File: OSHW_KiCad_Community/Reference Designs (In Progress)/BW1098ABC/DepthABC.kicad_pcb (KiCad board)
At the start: 4 copper layers, 150 x 65.2 mm, 118 parts, among them J1 Conn_02x05_Odd_Even, J13 DF23C-50DP-0.5V_92_, J2 FAN, J3 BW1099EMB_SoM, J4 Conn_02x05_Odd_Even, J5 USBC 3.1 Vertical, J6 26_pin_FFC, J7 26_pin_FFC, J9 26_pin_FFC, Q1 RK7002B, Q2 RK7002B, Q3 RK7002B, Q4 RK7002B, Q5 RK7002B, U1 2-bit bidirectional level shi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, U6 USB Type-C Switch, U7 USB Type-C Port Control

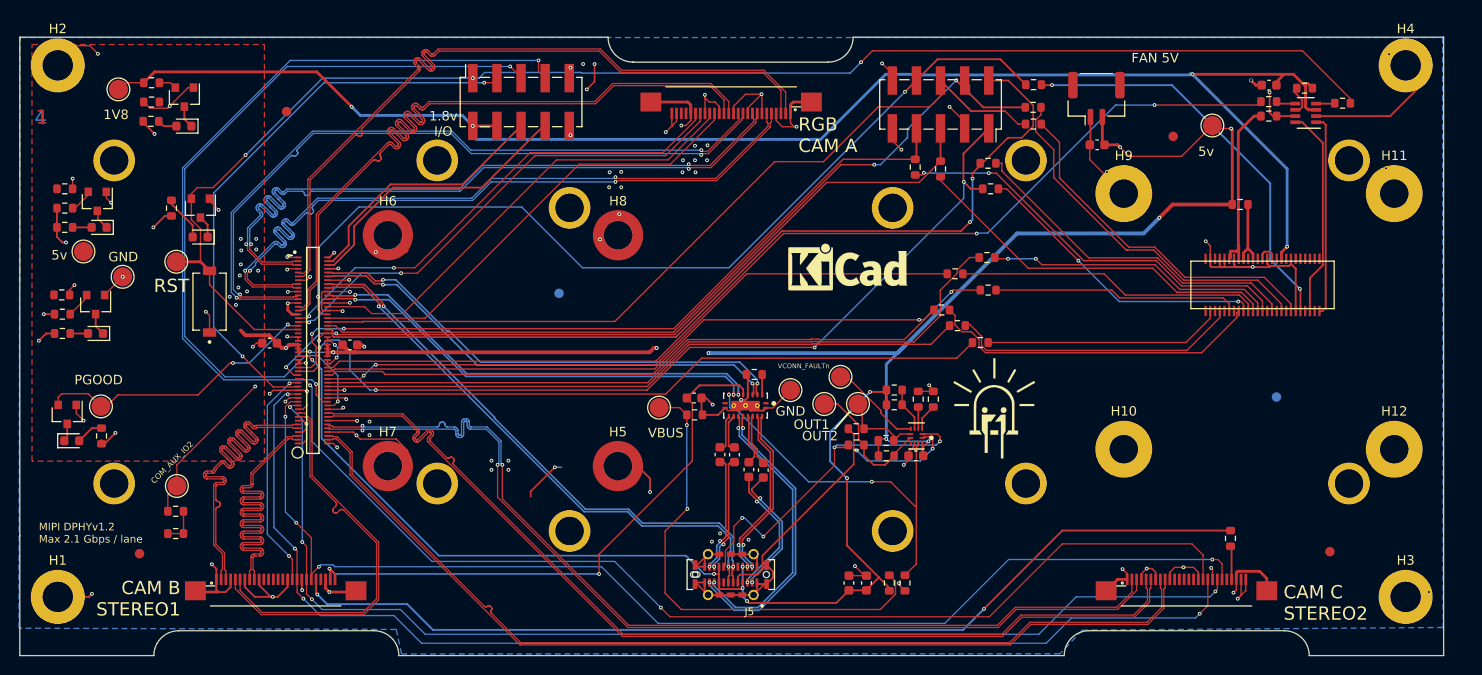
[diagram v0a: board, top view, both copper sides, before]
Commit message: skew
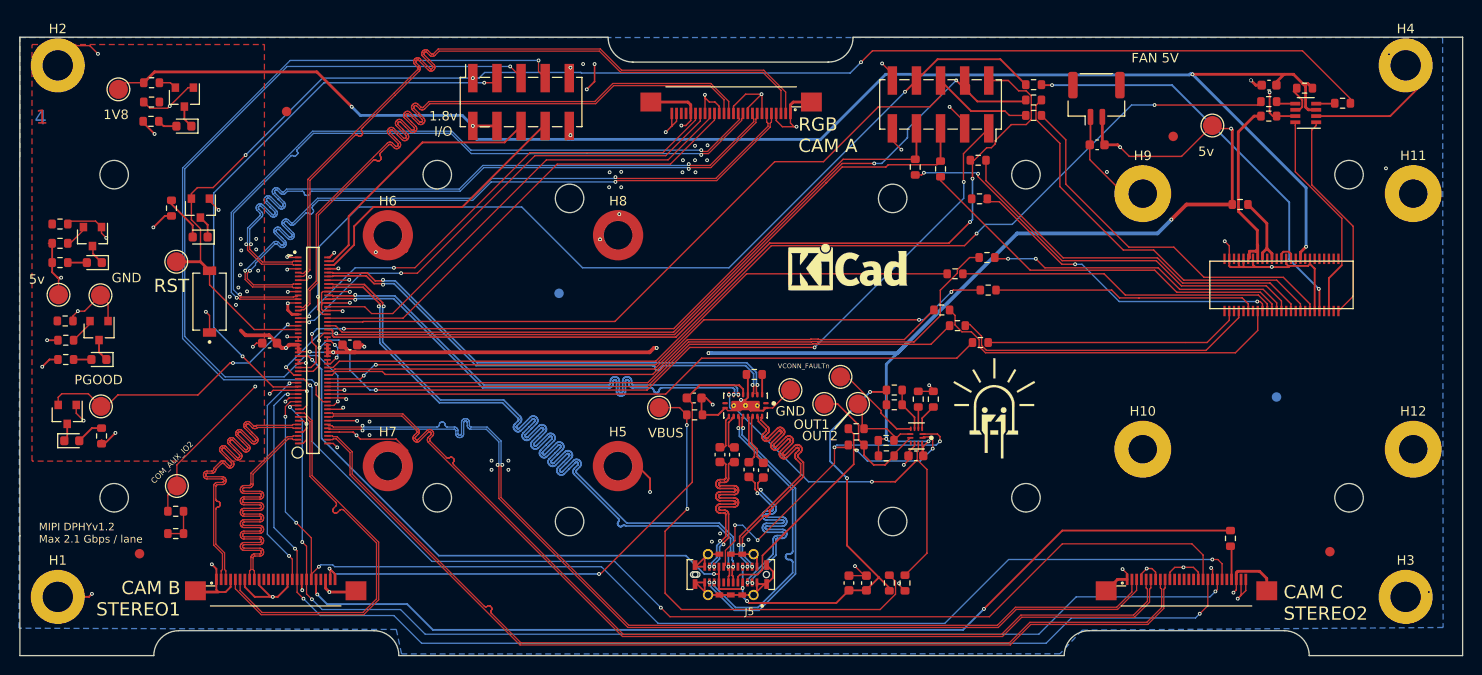
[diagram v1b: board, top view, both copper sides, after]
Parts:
- moved TP2 5.26 mm to (131.9, 119.9)
- moved R34 3.74 mm to (132.1, 112.5)
- moved D1 3.74 mm to (135.7, 116.5)
- moved Q1 3.74 mm to (135.5, 113.8)
- moved R1 3.74 mm to (132.1, 114.5)
- moved R2 3.74 mm to (132.1, 116.5)
- moved TP10 3.04 mm to (136.3, 120.0)
- moved Q4 2.77 mm to (136.2, 123.7)
- moved R30 2.77 mm to (132.7, 126.8)
- moved R33 2.77 mm to (132.6, 122.7)
- moved D4 2.77 mm to (136.2, 126.8)
- moved R29 2.77 mm to (132.7, 124.7)
- moved H10 2.00 mm to (246.2, 136.2)
- moved H11 2.00 mm to (274.7, 109.3)
- moved H12 2.00 mm to (274.7, 136.2)
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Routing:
- net USB_D_N: track 58.6 -> 85.0 mm
- net USB_D_P: track 59.0 -> 85.0 mm
- net /USBC&POWER/RXB_P: track 18.3 -> 31.4 mm
- net /USBC&POWER/RXB_N: track 18.3 -> 31.1 mm
- net /USBC&POWER/TXC_N: track 12.3 -> 21.1 mm
- net /USBC&POWER/TXC_P: track 12.3 -> 21.1 mm
- net /USBC&POWER/TXB_N: track 13.9 -> 21.1 mm
- net /USBC&POWER/TXB_P: track 14.4 -> 21.1 mm
- net GND: track 281.5 -> 287.8 mm, vias 102 -> 100
- net (no net): track 4.86 -> 0.00 mm, vias 1 -> 0
- net USB_TX_N: track 47.6 -> 52.2 mm
- net /USBC&POWER/P0.11: track 36.2 -> 40.4 mm
- net USB_TX_P: track 48.3 -> 52.1 mm
- net /USBC&POWER/P0.08: track 38.7 -> 41.6 mm
- net /USBC&POWER/P0.04: track 37.1 -> 40.0 mm
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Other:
- board size 150 x 65.2 mm -> 152 x 65.2 mm
